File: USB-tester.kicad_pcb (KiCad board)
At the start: 2 copper layers, 69.1 x 45.1 mm, 81 parts

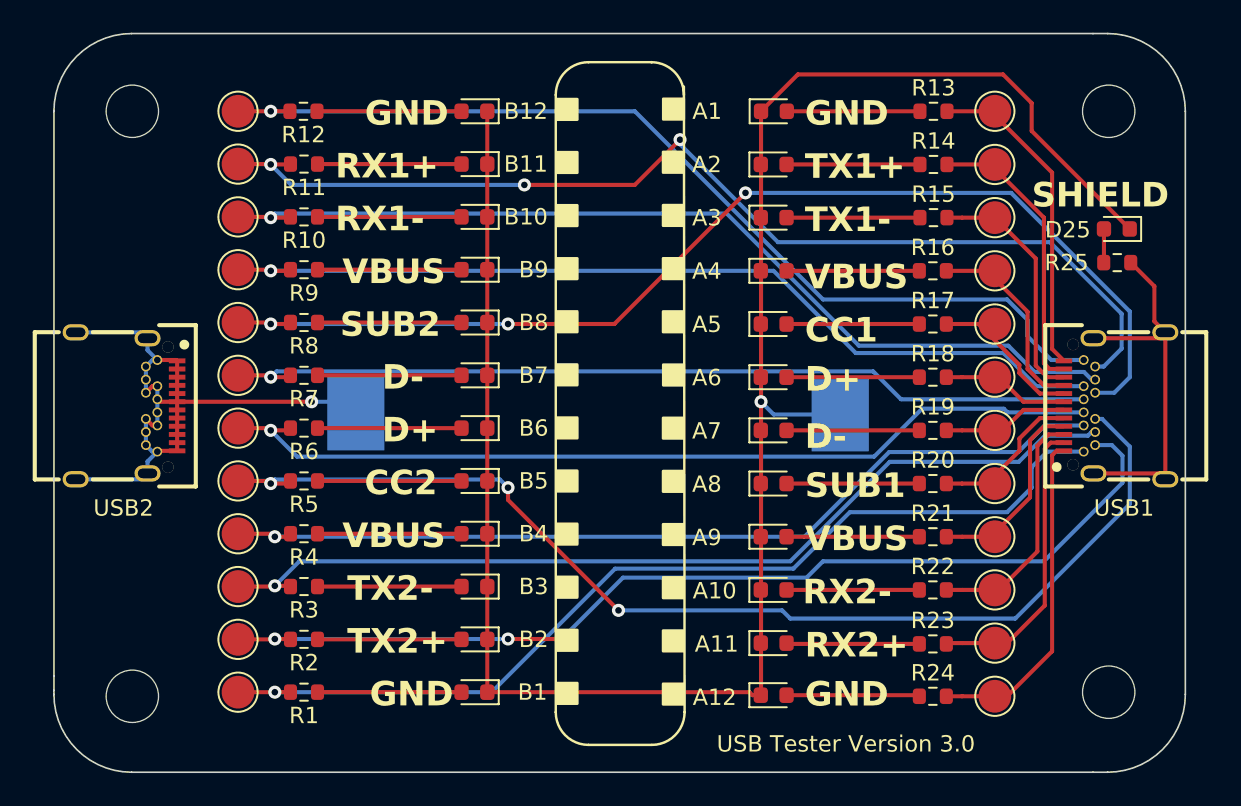
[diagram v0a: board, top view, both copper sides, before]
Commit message: Break out version
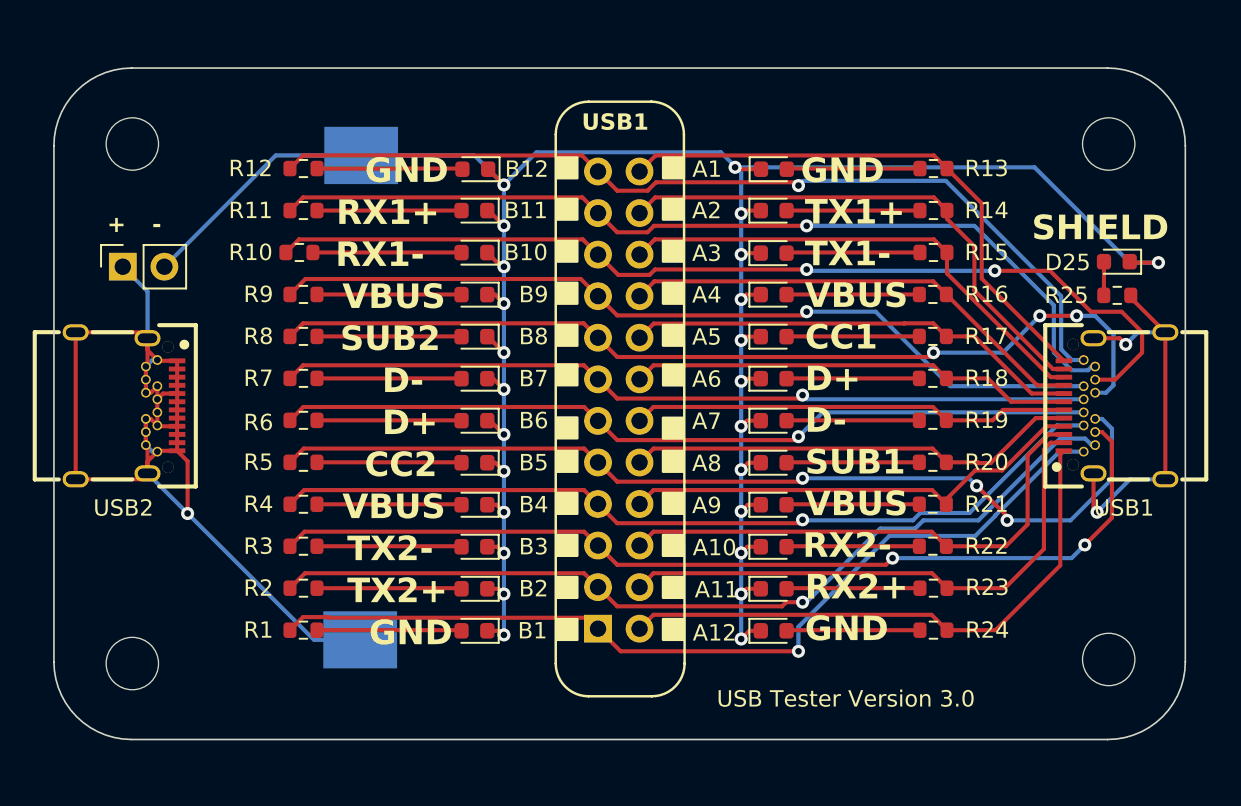
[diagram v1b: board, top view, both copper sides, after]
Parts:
- removed TP1, TP14, TP24, TP4: GND, TestPoint:TestPoint_Pad_D2.0mm
- removed TP10, TP19: D-, TestPoint:TestPoint_Pad_D2.0mm
- removed TP11: SUB1, TestPoint:TestPoint_Pad_D2.0mm
- removed TP12, TP16, TP21, TP8: VBUS, TestPoint:TestPoint_Pad_D2.0mm
- removed TP13, TP22: RX-, TestPoint:TestPoint_Pad_D2.0mm
- removed TP15, TP7: TX-, TestPoint:TestPoint_Pad_D2.0mm
- removed TP17: CC2, TestPoint:TestPoint_Pad_D2.0mm
- removed TP18, TP2: D+, TestPoint:TestPoint_Pad_D2.0mm
- removed TP20: SUB2, TestPoint:TestPoint_Pad_D2.0mm
- removed TP23, TP3: RX+, TestPoint:TestPoint_Pad_D2.0mm
- removed TP5, TP6: TX+, TestPoint:TestPoint_Pad_D2.0mm
- removed TP9: CC1, TestPoint:TestPoint_Pad_D2.0mm
- added J1: Conn_02x12_Odd_Even, Connector_PinSocket_2.54mm:PinSocket_2x12_P2.54mm_Vertical, F.Cu at (165.5, 114.2)
- added J2: Conn_01x02, Connector_PinSocket_2.54mm:PinSocket_1x02_P2.54mm_Vertical, F.Cu at (136.5, 92.1)
- moved BT2 14.5 mm to (151.0, 100.1), turned to 90 degrees
- moved R24 4.04 mm to (186.0, 114.3)
- moved A12 3.93 mm to (176.3, 114.4)
- moved R1 3.79 mm to (147.5, 114.3)
- moved B1 3.75 mm to (158.0, 114.4)
- moved B12 3.54 mm to (158.0, 86.1)
- moved A1 3.54 mm to (176.3, 86.1)
- moved R12 3.50 mm to (147.5, 86.1)
- moved R13 3.50 mm to (186.0, 86.1)
- moved R23 3.40 mm to (186.0, 111.8)
- moved A11 3.32 mm to (176.3, 111.8)
- moved R2 3.13 mm to (147.5, 111.8)
- moved B2 3.09 mm to (158.0, 111.8)
- moved B11 2.84 mm to (158.0, 88.7)
- moved R11 2.84 mm to (147.5, 88.7)
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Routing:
- net BAT-: track 121.5 -> 157.7 mm, vias 1 -> 25
- net A10_B: track 41.7 -> 72.3 mm
- net A7_A: track 7.80 -> 27.2 mm
- net A6_A: track 7.70 -> 26.9 mm
- net A8_A: track 9.24 -> 28.1 mm
- net A5_A: track 9.28 -> 27.8 mm
- net A3_A: track 14.9 -> 32.0 mm
- net A9_A: track 12.1 -> 28.9 mm
- net A4_A: track 12.0 -> 28.8 mm
- net A2_A: track 17.9 -> 33.9 mm
- net A10_A: track 15.0 -> 30.6 mm
- net A1_A: track 20.0 -> 35.2 mm
- net A11_A: track 17.5 -> 32.5 mm
- net A12_A: track 19.8 -> 34.2 mm
- net B8_A: track 71.2 -> 58.1 mm
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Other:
- board size 69.1 x 45.1 mm -> 69.1 x 41 mm
- board text added: "USB1"

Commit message: Adds images and README file
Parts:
- A1, A12, B1, B12: value LED -> LEDW
- A10, A11, A2, A3, B10, B11, B2, B3: value LED -> LEDY
- A4, A9, B4, B9: value LED -> LEDR
- A5, B5: value LED -> LEDB
- A6, A7, B6, B7: value LED -> LEDG
- A8, B8: value LED -> LEDV
- R1, R10, R11, R12, R13, R14, R15, R16, R17, R18, R19, R2, R20, R21, R22, R23, R24, R3, R4, R5, R6, R7, R8, R9: value 1000 -> 100
